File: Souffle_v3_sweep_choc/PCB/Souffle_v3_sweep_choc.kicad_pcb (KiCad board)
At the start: 2 copper layers, 137.2 x 114.5 mm, 84 parts, among them J1 LED, J2 4PIN, J3 OLED, J4 Conn_01x01_Female, J5 Conn_01x01_Female, SW1 SW_PUSH, SW10 SW_PUSH, SW11 SW_PUSH, SW12 SW_PUSH, SW13 SW_PUSH, SW14 SW_PUSH, SW15 SW_PUSH, SW16 SW_PUSH, SW17 SW_PUSH, SW18 SW_PUSH, SW19 SW_PUSH, SW2 SW_PUSH, SW20 SW_PUSH, SW21 SW_PUSH, SW22 SW_PUSH, SW23 SW_PUSH, SW24 SW_PUSH, SW25 SW_PUSH, SW25b1 RotaryEncoder_Switch, SW26 SW_PUSH, SW27 SW_PUSH, SW28 SW_PUSH, SW29 SW_PUSH, SW3 SW_PUSH, SW30 SW_PUSH, SW31 SW_SPDT, SW4 SW_PUSH, SW5 SW_PUSH, SW6 SW_PUSH, SW7 SW_PUSH, SW8 SW_PUSH, SW9 SW_PUSH, U1 ProMicro

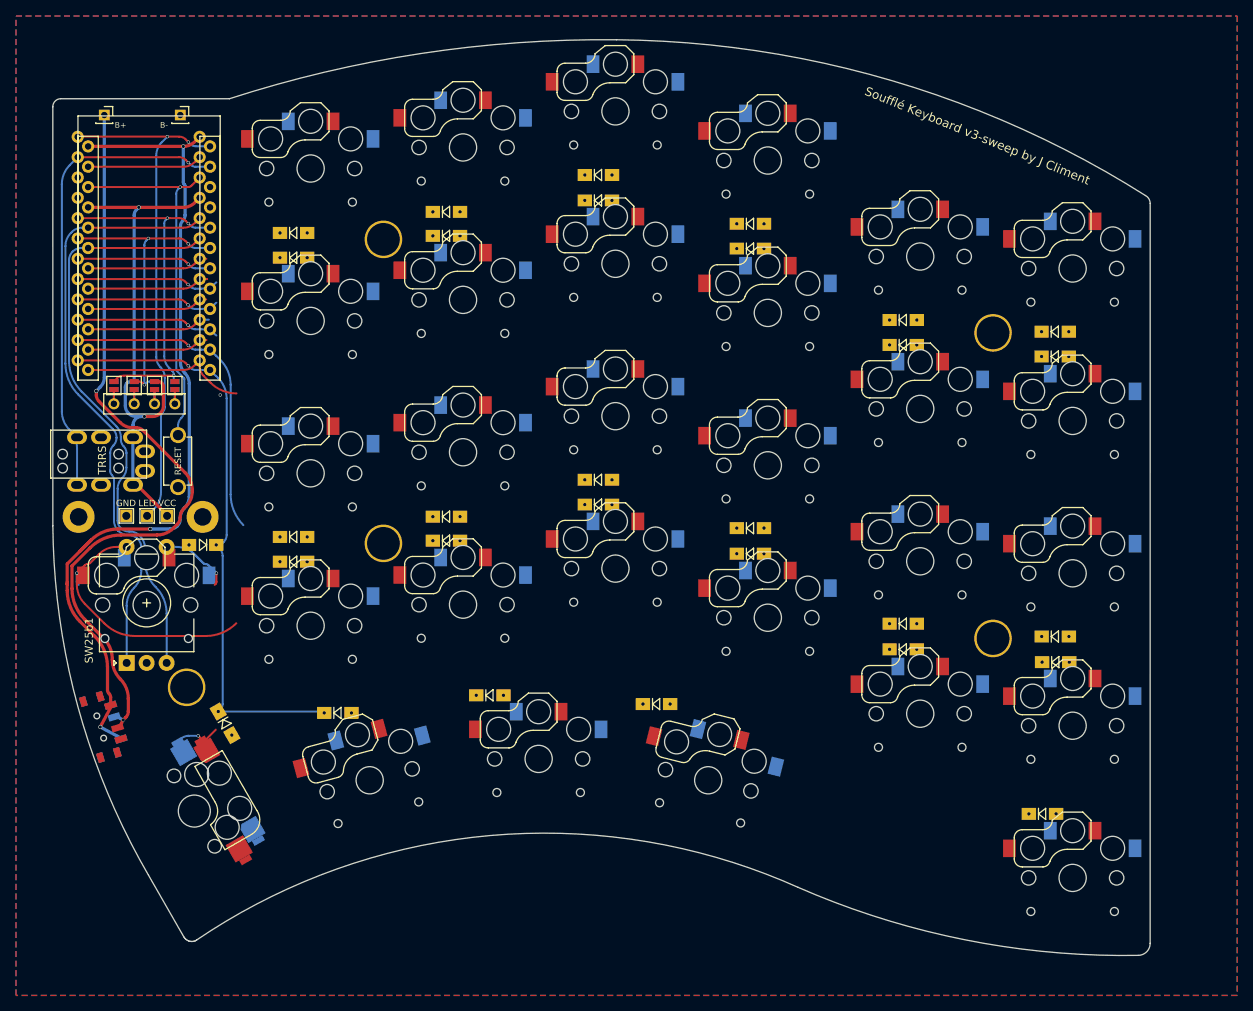
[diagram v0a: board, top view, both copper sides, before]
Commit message: Updated choc Soufflé.
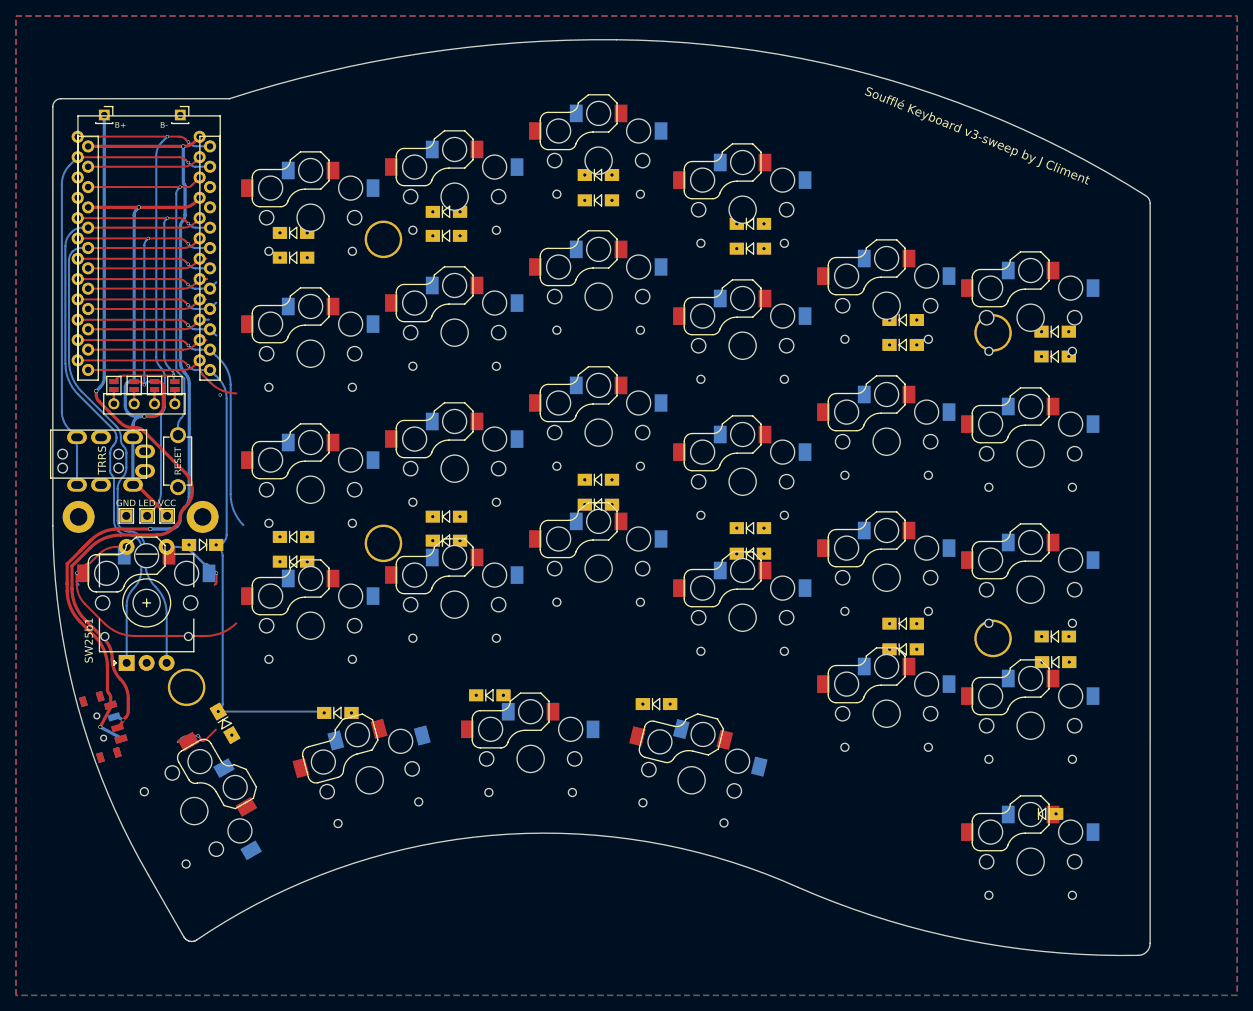
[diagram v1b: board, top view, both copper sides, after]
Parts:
- SW26: footprint SofleKeyboard-footprint:CherryMX_Hotswap_1.5_mod -> SofleKeyboard-footprint:Choc_Hotswap_Souffle
- moved SW6 8.09 mm to (196.1, 64.1)
- moved SW5 7.45 mm to (178.1, 62.6)
- moved SW4 6.91 mm to (160.1, 50.6)
- moved SW12 6.66 mm to (196.1, 81.1)
- moved SW3 6.50 mm to (142.1, 44.4)
- moved SW2 6.24 mm to (124.1, 48.9)
- moved SW1 6.15 mm to (106.1, 51.6)
- moved SW11 5.87 mm to (178.1, 79.6)
- moved SW18 5.64 mm to (196.1, 98.1)
- moved SW30 5.63 mm to (196.1, 132.1)
- moved SW24 5.25 mm to (196.1, 115.1)
- moved SW10 5.17 mm to (160.1, 67.6)
- moved SW17 4.67 mm to (178.1, 96.6)
- moved SW9 4.61 mm to (142.1, 61.4)
- moved SW8 4.23 mm to (124.1, 65.9)
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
